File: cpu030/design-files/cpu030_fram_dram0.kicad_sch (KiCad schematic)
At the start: 37 parts, among them J201 DRAM0SZ, J202 DRAM0 JTAG, U201 ATF1508AS, U202 CY7C1061GE (U16), U203 CY7C1061GE (L16), U204 SIMM72-0A, U205 SIMM72-0B, U206 MC74ACT05DG

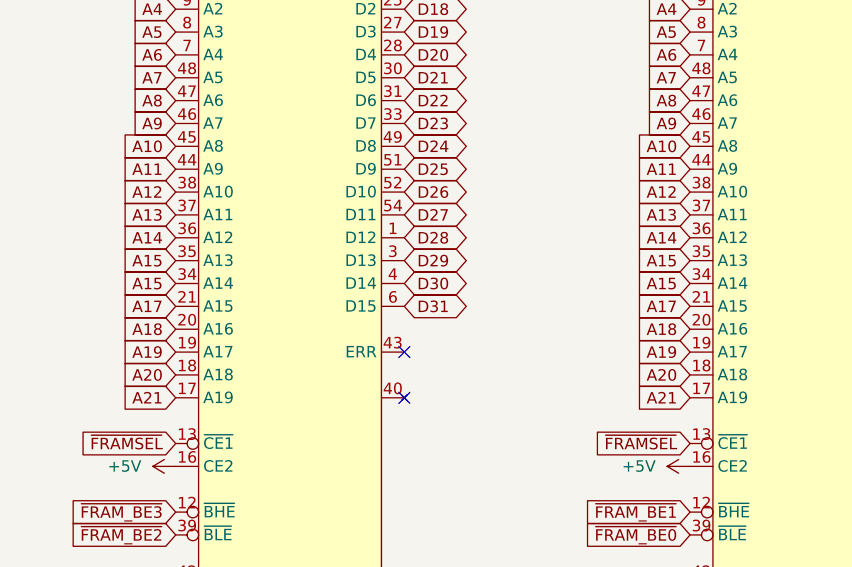
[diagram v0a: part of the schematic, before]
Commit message: Fix a mistake!  A15 was connected to the SRAM twice, and A16 wasn't connected at all!  I guess hand-routing is the way to go after all!
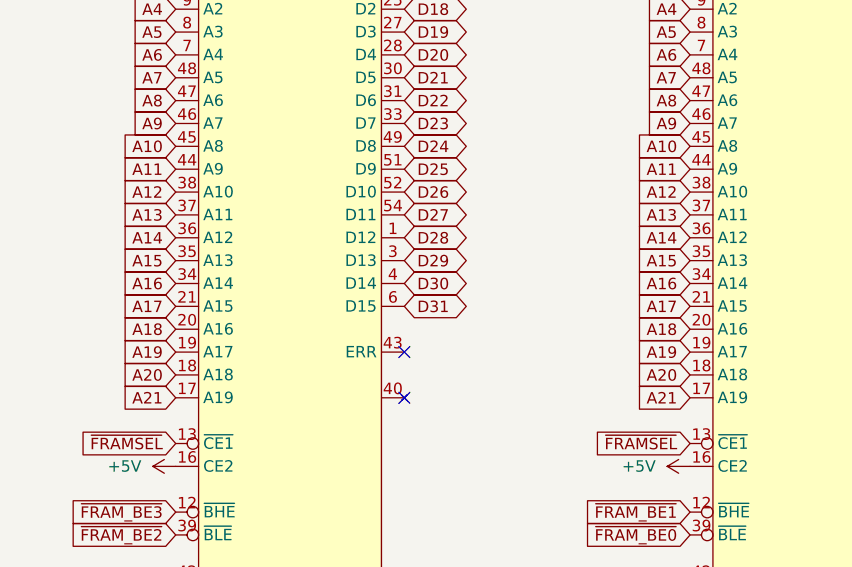
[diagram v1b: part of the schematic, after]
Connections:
- net A15: no longer U202.34 (A14), U203.34 (A14)
- net A16: now also U202.34 (A14), U203.34 (A14)
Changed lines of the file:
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@@
 		)
 	)
-	(global_label "A15"
+	(global_label "A16"
 		(shape input)
 		(at 25.4 62.23 180)
@@
 		)
 	)
-	(global_label "A15"
+	(global_label "A16"
 		(shape input)
 		(at 82.55 62.23 180)
